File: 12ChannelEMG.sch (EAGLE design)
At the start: 133 parts

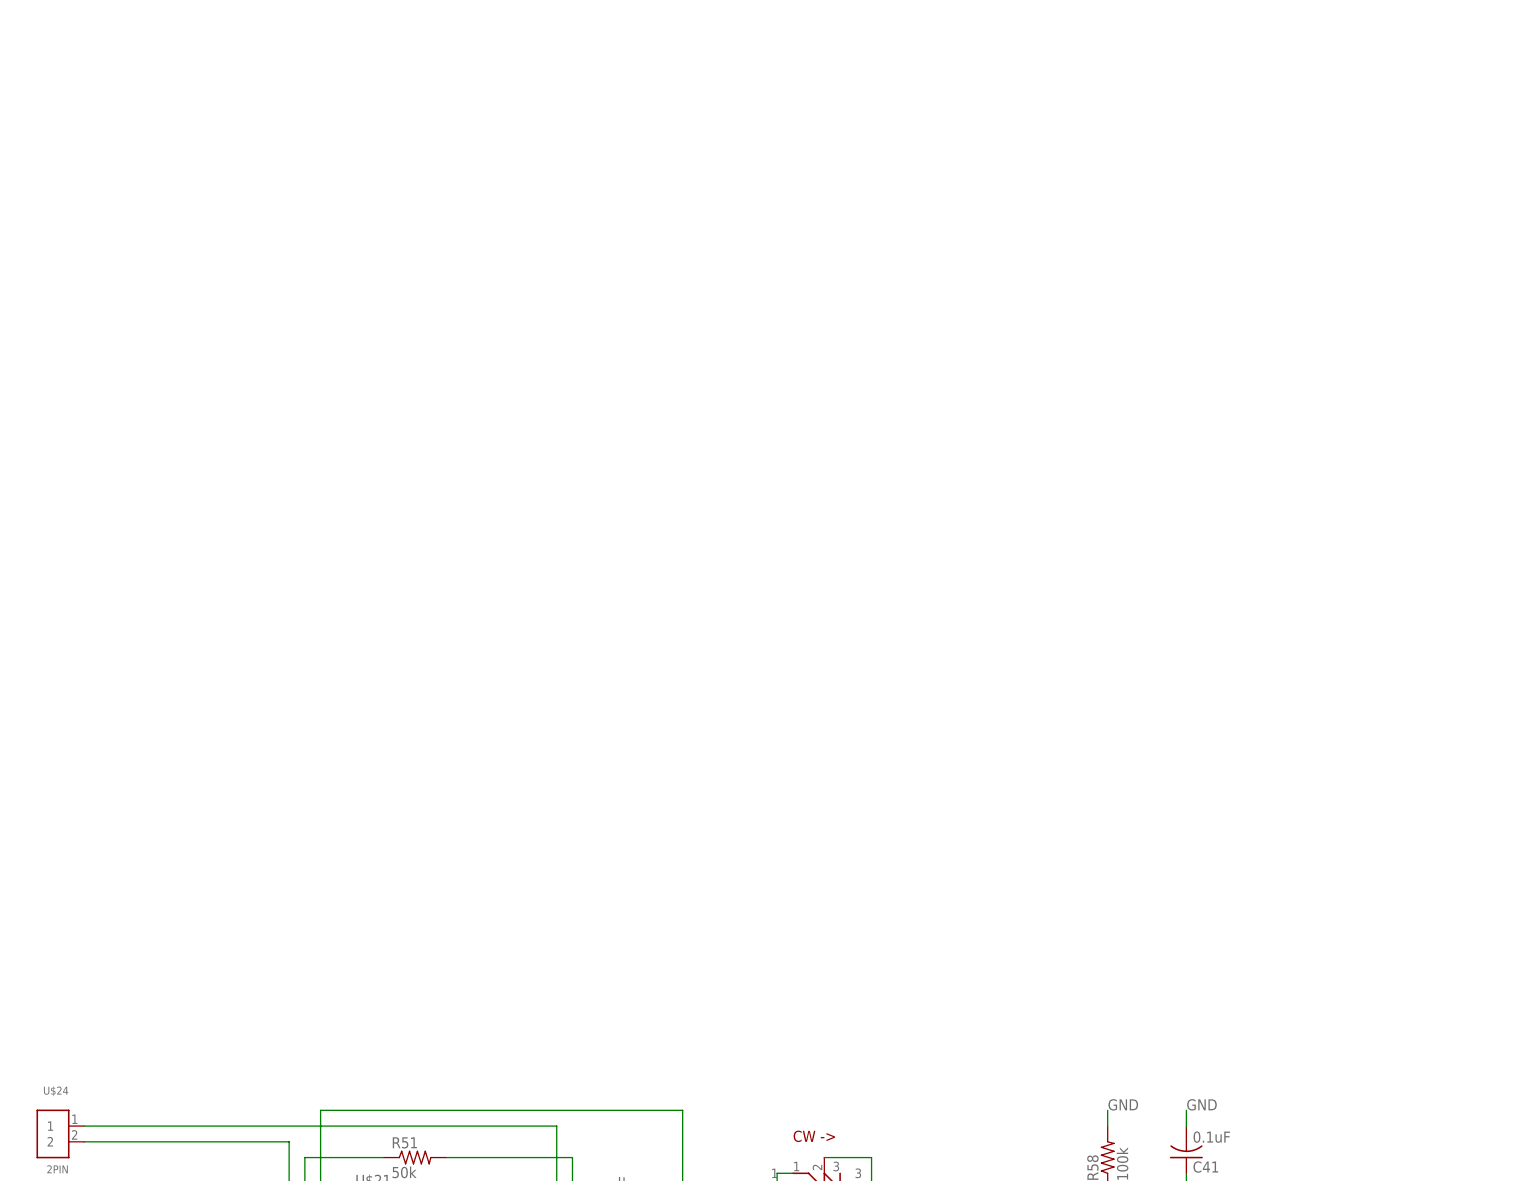
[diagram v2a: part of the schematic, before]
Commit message: Channel 9
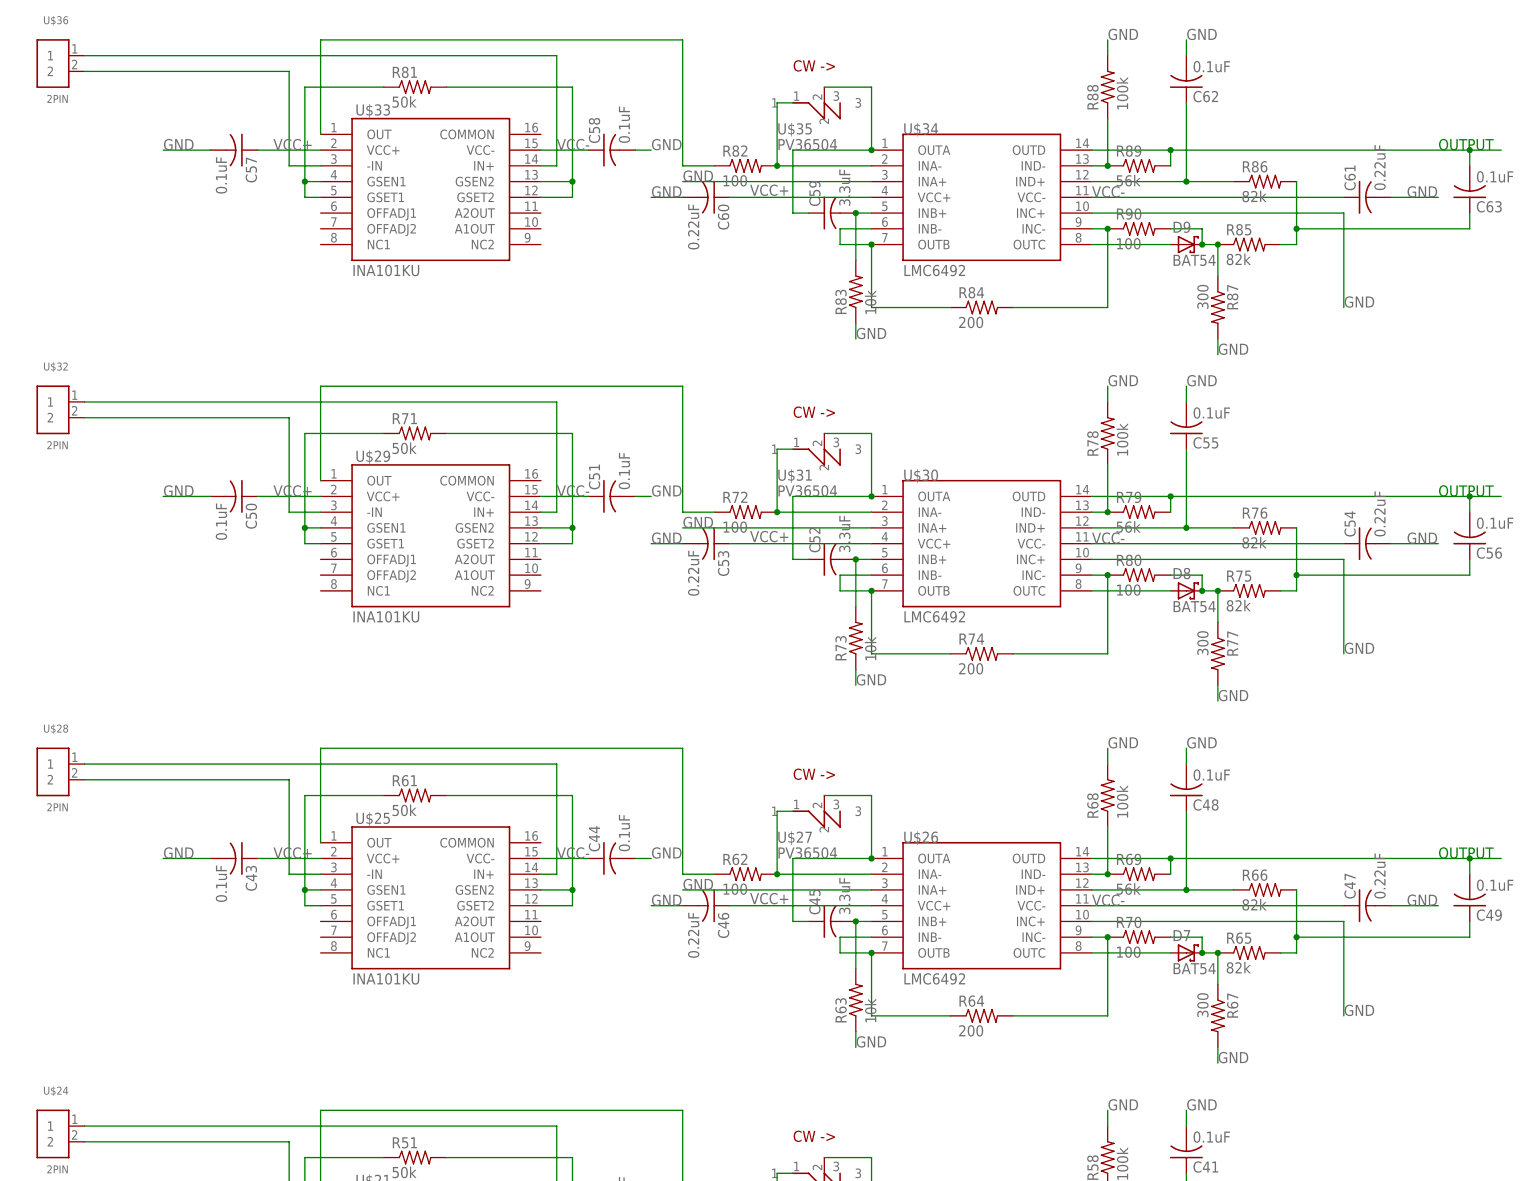
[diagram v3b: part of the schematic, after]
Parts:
- added C43, C44, C48, C49, C50, C51, C55, C56, C57, C58, C62, C63: 0.1uF, resistor:C-USC1206K
- added C45, C52, C59: 3.3uF, resistor:C-USC1206K
- added C46, C47, C53, C54, C60, C61: 0.22uF, rcl:C-USC0603K
- added D7, D8, D9: BAT54, diode:BAT54
- added R61, R71, R81: 50k, rcl:R-US_R0805
- added R62, R70, R72, R80, R82, R90: 100, resistor:R-US_R0603
- added R63, R73, R83: 10k, rcl:R-US_R0603
- added R64, R74, R84: 200, rcl:R-US_R0603
- added R65, R66, R75, R76, R85, R86: 82k, resistor:R-US_R0603
- added R67, R77, R87: 300, resistor:R-US_R0603
- added R68, R78, R88: 100k, resistor:R-US_R0603
- added R69, R79, R89: 56k, resistor:R-US_R0603
- added U$25, U$29, U$33: INA101KU, 12-ChannelEMG:INA101KUINA101KU
- added U$26, U$30, U$34: LMC6492, 12-ChannelEMG:LMC6492
- added U$27, U$31, U$35: PV36504, 12-ChannelEMG:PV36
- added U$28, U$32, U$36: 2PIN, 12-ChannelEMG:2PIN
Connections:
- new net N$100: U$25.-IN, U$28.2
- new net N$101: R62.2, U$26.INA-, U$27.1
- new net N$102: R62.1, U$25.OUT
- new net N$103: C45.1, U$26.OUTA, U$27.2
- new net N$104: C45.2, R63.2, U$26.INB+
- new net N$105: R64.1, U$26.INB-, U$26.OUTB
- new net N$106: R64.2, R70.1, U$26.INC-
- new net N$107: D7.A, U$26.OUTC
- new net N$108: C48.1, R66.1, U$26.IND+
- new net N$109: D7.C, R65.1, R67.1, R70.2
- new net N$110: C49.2, R69.2, U$26.OUTD
- new net N$111: R68.1, R69.1, U$26.IND-
- new net N$112: C49.1, R65.2, R66.2
- new net N$113: R61.1, U$25.GSEN1, U$25.GSET1
- new net N$114: U$25.IN+, U$28.1
- new net N$115: R71.2, U$29.GSEN2, U$29.GSET2
- new net N$116: U$29.-IN, U$32.2
- new net N$117: R72.2, U$30.INA-, U$31.1
- new net N$118: R72.1, U$29.OUT
- new net N$119: C52.1, U$30.OUTA, U$31.2
- new net N$120: C52.2, R73.2, U$30.INB+
- new net N$121: R74.1, U$30.INB-, U$30.OUTB
- new net N$122: R74.2, R80.1, U$30.INC-
- new net N$123: D8.A, U$30.OUTC
- new net N$124: C55.1, R76.1, U$30.IND+
- new net N$125: D8.C, R75.1, R77.1, R80.2
- new net N$126: C56.2, R79.2, U$30.OUTD
- new net N$127: R78.1, R79.1, U$30.IND-
- new net N$128: C56.1, R75.2, R76.2
- new net N$129: R71.1, U$29.GSEN1, U$29.GSET1
- new net N$130: U$29.IN+, U$32.1
- new net N$131: R81.2, U$33.GSEN2, U$33.GSET2
- new net N$132: U$33.-IN, U$36.2
- new net N$133: R82.2, U$34.INA-, U$35.1
- new net N$134: R82.1, U$33.OUT
- new net N$135: C59.1, U$34.OUTA, U$35.2
- new net N$136: C59.2, R83.2, U$34.INB+
- new net N$137: R84.1, U$34.INB-, U$34.OUTB
- new net N$138: R84.2, R90.1, U$34.INC-
- new net N$139: D9.A, U$34.OUTC
- new net N$140: C62.1, R86.1, U$34.IND+
- new net N$141: D9.C, R85.1, R87.1, R90.2
- new net N$142: C63.2, R89.2, U$34.OUTD
- new net N$143: R88.1, R89.1, U$34.IND-
- new net N$144: C63.1, R85.2, R86.2
- new net N$145: R81.1, U$33.GSEN1, U$33.GSET1
- new net N$146: U$33.IN+, U$36.1
- new net N$99: R61.2, U$25.GSEN2, U$25.GSET2
- net GND: now also C43.2, C44.2, C46.2, C47.2, C48.2, C50.2, C51.2, C53.2, C54.2, C55.2, C57.2, C58.2, C60.2, C61.2, C62.2, R63.1, R67.2, R68.2, R73.1, R77.2, R78.2, R83.1, R87.2, R88.2, U$26.INA+, U$26.INC+, U$30.INA+, U$30.INC+, U$34.INA+, U$34.INC+
- net VCC+: now also C43.1, C46.1, C50.1, C53.1, C57.1, C60.1, U$25.VCC+, U$26.VCC+, U$29.VCC+, U$30.VCC+, U$33.VCC+, U$34.VCC+
- net VCC-: now also C44.1, C47.1, C51.1, C54.1, C58.1, C61.1, U$25.VCC-, U$26.VCC-, U$29.VCC-, U$30.VCC-, U$33.VCC-, U$34.VCC-

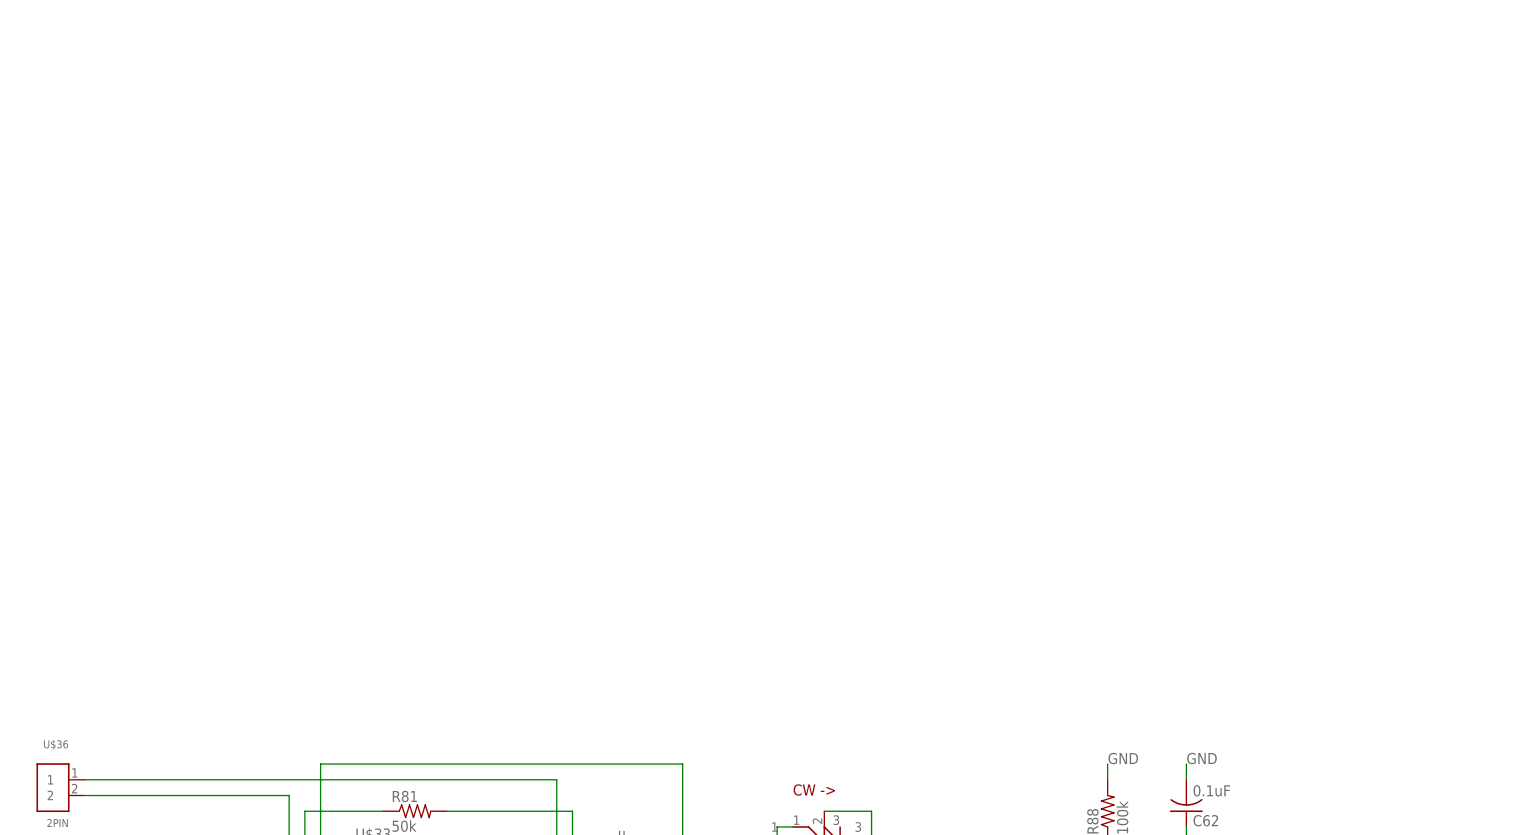
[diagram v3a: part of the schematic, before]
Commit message: Channel 11
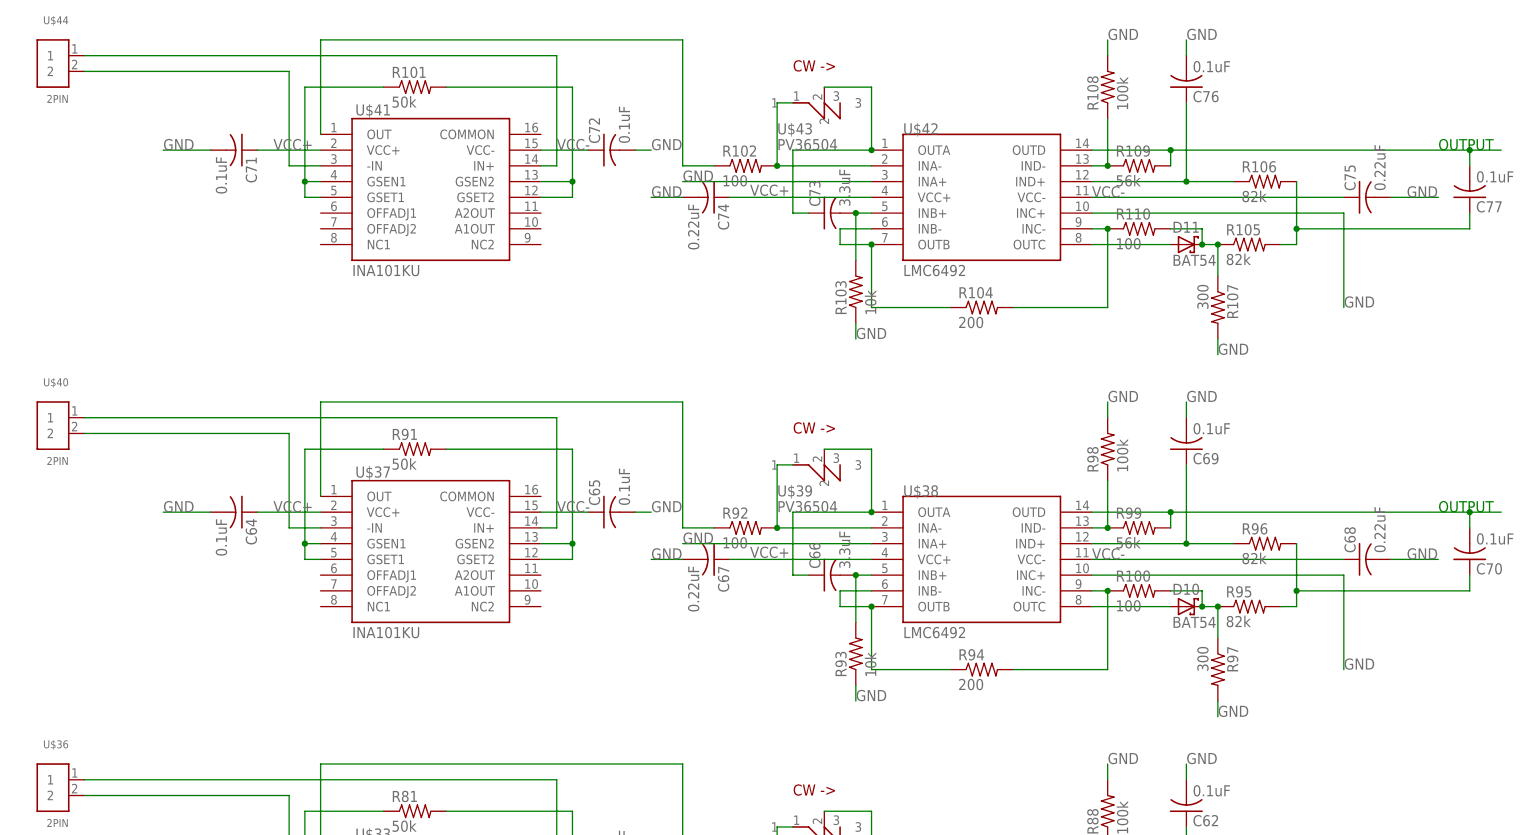
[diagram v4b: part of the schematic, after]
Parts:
- added C64, C65, C69, C70, C71, C72, C76, C77: 0.1uF, resistor:C-USC1206K
- added C66, C73: 3.3uF, resistor:C-USC1206K
- added C67, C68, C74, C75: 0.22uF, rcl:C-USC0603K
- added D10, D11: BAT54, diode:BAT54
- added R100, R102, R110, R92: 100, resistor:R-US_R0603
- added R101, R91: 50k, rcl:R-US_R0805
- added R103, R93: 10k, rcl:R-US_R0603
- added R104, R94: 200, rcl:R-US_R0603
- added R105, R106, R95, R96: 82k, resistor:R-US_R0603
- added R107, R97: 300, resistor:R-US_R0603
- added R108, R98: 100k, resistor:R-US_R0603
- added R109, R99: 56k, resistor:R-US_R0603
- added U$37, U$41: INA101KU, 12-ChannelEMG:INA101KUINA101KU
- added U$38, U$42: LMC6492, 12-ChannelEMG:LMC6492
- added U$39, U$43: PV36504, 12-ChannelEMG:PV36
- added U$40, U$44: 2PIN, 12-ChannelEMG:2PIN
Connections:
- new net N$147: R91.2, U$37.GSEN2, U$37.GSET2
- new net N$148: U$37.-IN, U$40.2
- new net N$149: R92.2, U$38.INA-, U$39.1
- new net N$150: R92.1, U$37.OUT
- new net N$151: C66.1, U$38.OUTA, U$39.2
- new net N$152: C66.2, R93.2, U$38.INB+
- new net N$153: R94.1, U$38.INB-, U$38.OUTB
- new net N$154: R100.1, R94.2, U$38.INC-
- new net N$155: D10.A, U$38.OUTC
- new net N$156: C69.1, R96.1, U$38.IND+
- new net N$157: D10.C, R100.2, R95.1, R97.1
- new net N$158: C70.2, R99.2, U$38.OUTD
- new net N$159: R98.1, R99.1, U$38.IND-
- new net N$160: C70.1, R95.2, R96.2
- new net N$161: R91.1, U$37.GSEN1, U$37.GSET1
- new net N$162: U$37.IN+, U$40.1
- new net N$163: R101.2, U$41.GSEN2, U$41.GSET2
- new net N$164: U$41.-IN, U$44.2
- new net N$165: R102.2, U$42.INA-, U$43.1
- new net N$166: R102.1, U$41.OUT
- new net N$167: C73.1, U$42.OUTA, U$43.2
- new net N$168: C73.2, R103.2, U$42.INB+
- new net N$169: R104.1, U$42.INB-, U$42.OUTB
- new net N$170: R104.2, R110.1, U$42.INC-
- new net N$171: D11.A, U$42.OUTC
- new net N$172: C76.1, R106.1, U$42.IND+
- new net N$173: D11.C, R105.1, R107.1, R110.2
- new net N$174: C77.2, R109.2, U$42.OUTD
- new net N$175: R108.1, R109.1, U$42.IND-
- new net N$176: C77.1, R105.2, R106.2
- new net N$177: R101.1, U$41.GSEN1, U$41.GSET1
- new net N$178: U$41.IN+, U$44.1
- net GND: now also C64.2, C65.2, C67.2, C68.2, C69.2, C71.2, C72.2, C74.2, C75.2, C76.2, R103.1, R107.2, R108.2, R93.1, R97.2, R98.2, U$38.INA+, U$38.INC+, U$42.INA+, U$42.INC+
- net VCC+: now also C64.1, C67.1, C71.1, C74.1, U$37.VCC+, U$38.VCC+, U$41.VCC+, U$42.VCC+
- net VCC-: now also C65.1, C68.1, C72.1, C75.1, U$37.VCC-, U$38.VCC-, U$41.VCC-, U$42.VCC-
